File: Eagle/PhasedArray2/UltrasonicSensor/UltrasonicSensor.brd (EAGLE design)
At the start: 100 x 80 mm, 103 parts

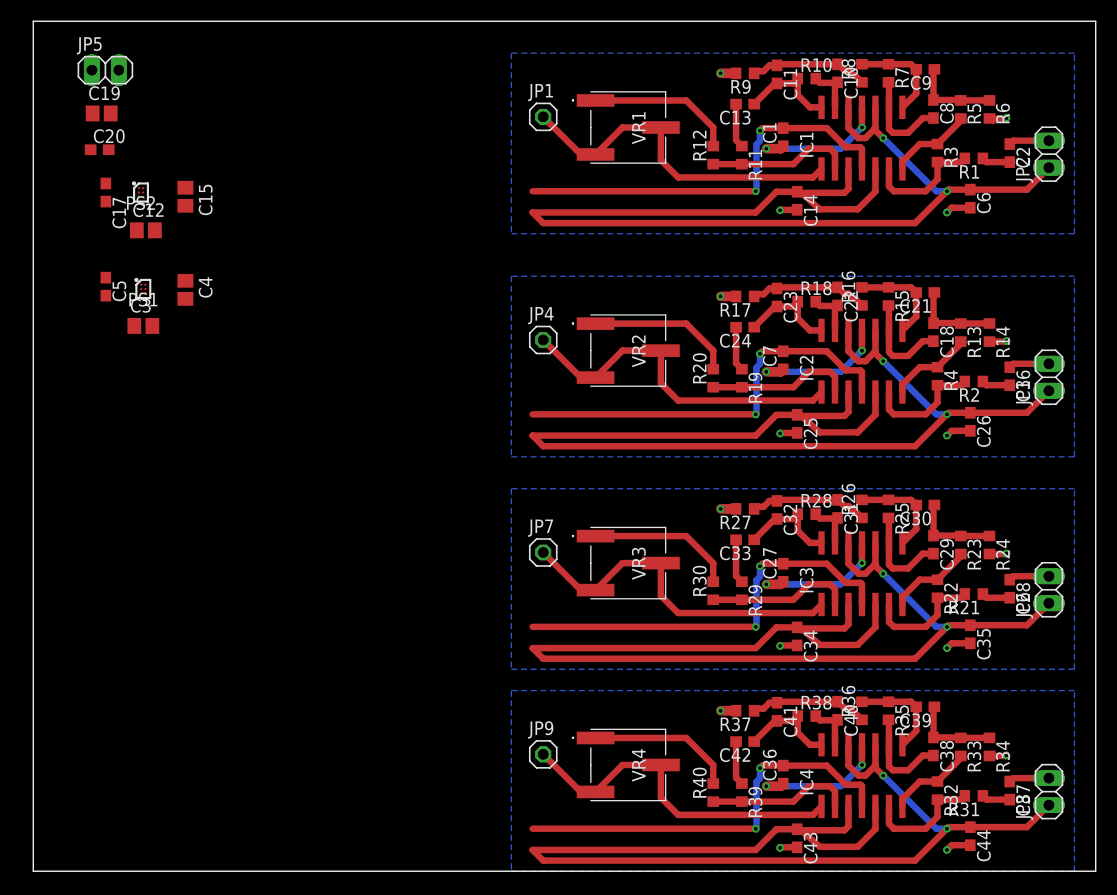
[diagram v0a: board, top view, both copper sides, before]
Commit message: Add files via upload
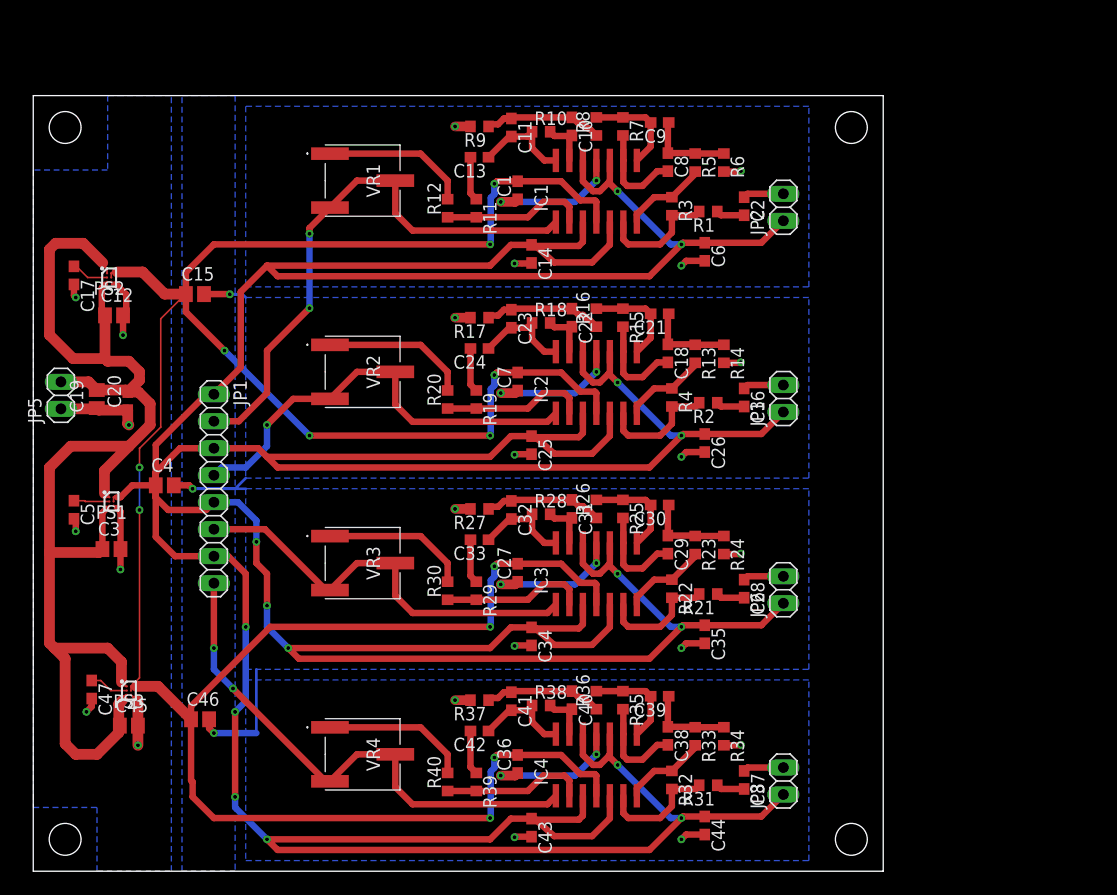
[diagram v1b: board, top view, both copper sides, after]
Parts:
- removed JP4, JP7, JP9: (no value), pinhead:1X01
- added C45, C46: 10u, rcl:C2012
- added C47: 1000p, rcl:C1608
- added PS3: ADP7112ACBZ-5.0-R7, ADP7112ACBZ-3.3-R7:BGA6C40P2X3_95X116X56
- JP1: device pinhead:1X01 -> pinhead:1X08
- moved JP1 46.8 mm to (17.0, 36.0), turned to 270 degrees
- moved JP5 30.9 mm to (2.60, 44.8), turned to 90 degrees
- moved C19 26.9 mm to (5.98, 44.4), turned to 90 degrees
- moved C14 25.5 mm to (46.9, 58.1)
- moved C8 25.5 mm to (59.7, 66.7)
- moved C1 25.5 mm to (45.6, 64.1)
- moved C10 25.5 mm to (50.7, 70.1)
- moved C11 25.5 mm to (45.0, 70.0)
- moved C13 25.5 mm to (42.0, 67.2)
- moved C2 25.5 mm to (66.9, 62.6)
- moved C6 25.5 mm to (63.2, 58.3)
- moved IC1 25.5 mm to (53.0, 64.0)
- moved R1 25.5 mm to (63.5, 62.1)
- moved R10 25.5 mm to (47.8, 69.6)
- moved R11 25.5 mm to (41.7, 62.4)
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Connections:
- new net N$59: C47.1, PS3.B1
- net +9V: now also C45.1, PS3.A1, PS3.C1
- net AGND: now also C46.2
- net GND: now also C45.2, C47.2, PS3.C2
- net N$16: now also JP1.2; no longer JP1.1
- net N$29: now also JP1.4; no longer JP4.1
- net N$44: now also JP1.6; no longer JP7.1
- net N$58: now also JP1.8; no longer JP9.1
- net VCC: now also C46.1, PS3.A2, PS3.B2
- net VCC/2: now also JP1.1, JP1.3, JP1.5, JP1.7
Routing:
- net +9V: track 0.00 -> 119.3 mm
- net VCC: track 157.1 -> 263.6 mm, vias 8 -> 12
- net VCC/2: track 444.3 -> 550.4 mm, vias 8 -> 15
- net AGND: track 82.0 -> 112.5 mm, vias 24 -> 27
- net GND: track 0.00 -> 29.2 mm, vias 0 -> 7
- net N$16: track 32.8 -> 52.4 mm, vias 0 -> 2
- net N$58: track 32.8 -> 49.8 mm, vias 0 -> 2
- net N$29: track 32.8 -> 41.5 mm, vias 0 -> 1
- net N$44: track 32.8 -> 39.7 mm
- net N$59: track 0.00 -> 3.69 mm
- net N$34: track 0.00 -> 3.54 mm
- net N$6: track 0.00 -> 3.36 mm
- added copper zone on layer 16, net GND
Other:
- board size 100 x 80 mm -> 80 x 73 mm
